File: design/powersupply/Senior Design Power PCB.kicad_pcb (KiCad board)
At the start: 2 copper layers, 70.1 x 32 mm, 16 parts, among them U1 VSSOP-10_3x3mm_P0.5mm, U2 TO-263-5_TabPin3

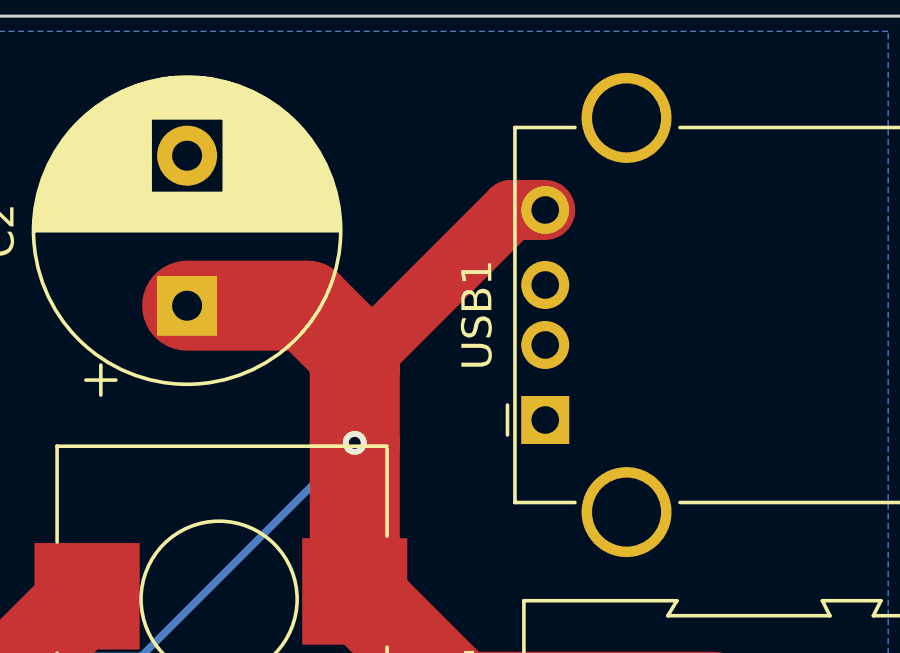
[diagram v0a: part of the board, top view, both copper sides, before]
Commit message: updated board layout
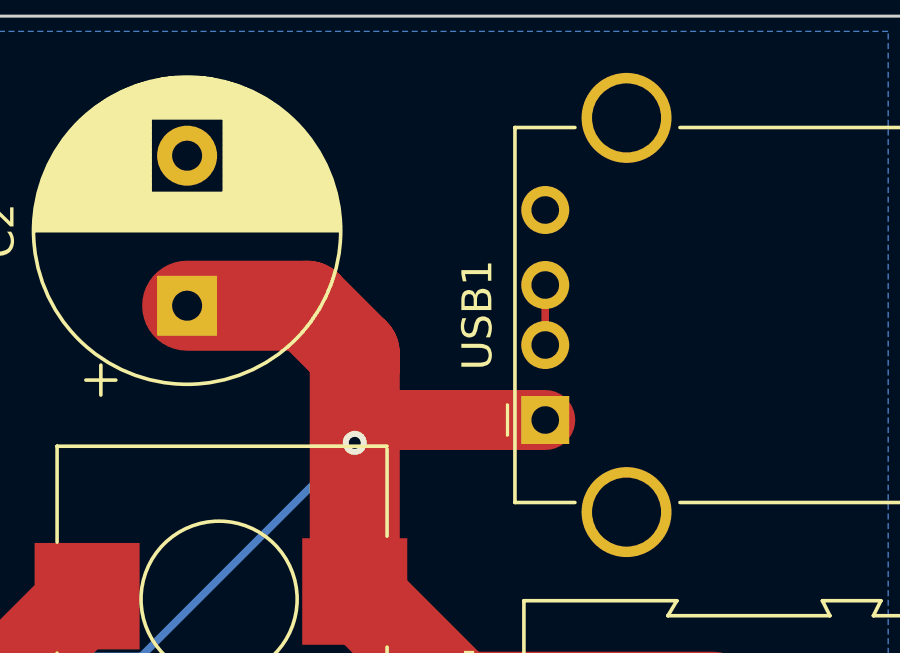
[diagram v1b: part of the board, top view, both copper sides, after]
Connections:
- USB1 pad 1: B- -> 5V
- USB1 pad 4: 5V -> B-
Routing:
- net (no net): track 52.8 -> 54.8 mm
- net 5V: track 103.9 -> 102.0 mm
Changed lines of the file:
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@@
-(kicad_pcb (version 20171130) (host pcbnew "(5.1.4)-1")
+(kicad_pcb (version 20171130) (host pcbnew 5.1.4-e60b266~84~ubuntu18.04.1)
   (general
     (thickness 1.6)
     (drawings 15)
-    (tracks 155)
+    (tracks 156)
     (zones 0)
     (modules 16)
@@
     (mod_text_size 1 1)
     (mod_text_width 0.15)
-    (pad_size 2 2)
-    (pad_drill 1)
+    (pad_size 1.6 1.6)
+    (pad_drill 0.92)
     (pad_to_mask_clearance 0.051)
     (solder_mask_min_width 0.25)
@@
     (fp_line (start 10.25 4.74) (end 11.25 4.74) (layer F.CrtYd) (width 0.05))
     (pad 4 thru_hole circle (at 7 0 90) (size 1.6 1.6) (drill 0.92) (layers *.Cu *.Mask)
-      (net 4 5V))
+      (net 1 B-))
     (pad 3 thru_hole circle (at 4.5 0 90) (size 1.6 1.6) (drill 0.92) (layers *.Cu *.Mask))
     (pad 2 thru_hole circle (at 2.5 0 90) (size 1.6 1.6) (drill 0.92) (layers *.Cu *.Mask))
     (pad 1 thru_hole rect (at 0 0 90) (size 1.6 1.6) (drill 0.92) (layers *.Cu *.Mask)
-      (net 1 B-))
+      (net 4 5V))
     (pad 5 thru_hole circle (at -3.07 2.71 90) (size 3 3) (drill 2.3) (layers *.Cu *.Mask)
       (net 1 B-))
@@
   (segment (start 54.863 44.197) (end 61.436 37.624) (width 3) (layer F.Cu) (net 0))
   (segment (start 52.427 44.197) (end 54.863 44.197) (width 3) (layer F.Cu) (net 0))
+  (segment (start 76.708 29.25) (end 76.708 27.25) (width 0.25) (layer F.Cu) (net 0))
   (via (at 48.26 24.13) (size 0.8) (drill 0.4) (layers F.Cu B.Cu) (net 1))
   (via (at 48.26 25.4) (size 0.8) (drill 0.4) (layers F.Cu B.Cu) (net 1))
@@
   (segment (start 73.867 40.974) (end 82.296 40.974) (width 3) (layer F.Cu) (net 4))
   (segment (start 70.358 37.465) (end 73.867 40.974) (width 3) (layer F.Cu) (net 4))
-  (segment (start 75.57663 24.75) (end 70.358 29.96863) (width 2) (layer F.Cu) (net 4))
-  (segment (start 76.708 24.75) (end 75.57663 24.75) (width 2) (layer F.Cu) (net 4))
   (segment (start 70.358 37.465) (end 70.358 32.512) (width 3) (layer F.Cu) (net 4))
   (segment (start 70.358 29.528) (end 70.358 29.96863) (width 3) (layer F.Cu) (net 4))
@@
   (segment (start 43.942 39.624) (end 39.878 43.688) (width 0.25) (layer B.Cu) (net 4))
   (segment (start 64.77 26.69) (end 64.77 27.94) (width 0.25) (layer F.Cu) (net 4))
+  (segment (start 71.12 31.75) (end 70.358 32.512) (width 2) (layer F.Cu) (net 4))
+  (segment (start 76.708 31.75) (end 71.12 31.75) (width 2) (layer F.Cu) (net 4))
   (segment (start 27.6 37.846) (end 27.6 37.346) (width 0.2) (layer F.Cu) (net 5))
   (segment (start 39.5875 25.146) (end 39.5875 28.7385) (width 0.25) (layer F.Cu) (net 5))
